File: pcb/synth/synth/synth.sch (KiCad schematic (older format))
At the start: 3 parts, among them J1 Screw_Terminal_01x06, J2 AudioJack2, J3 Conn_02x07_Odd_Even

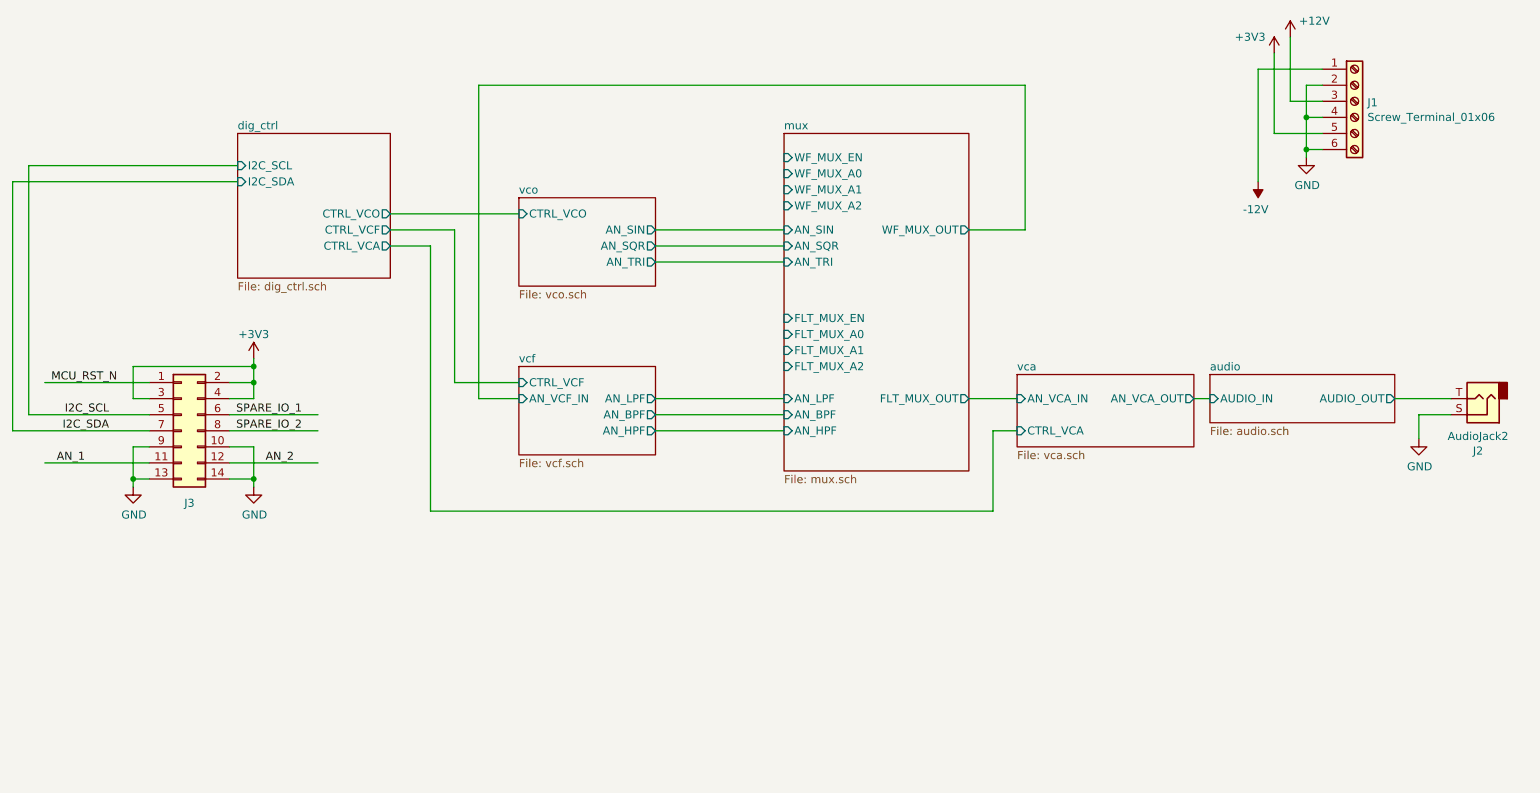
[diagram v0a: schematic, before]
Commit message: inital synth schematic
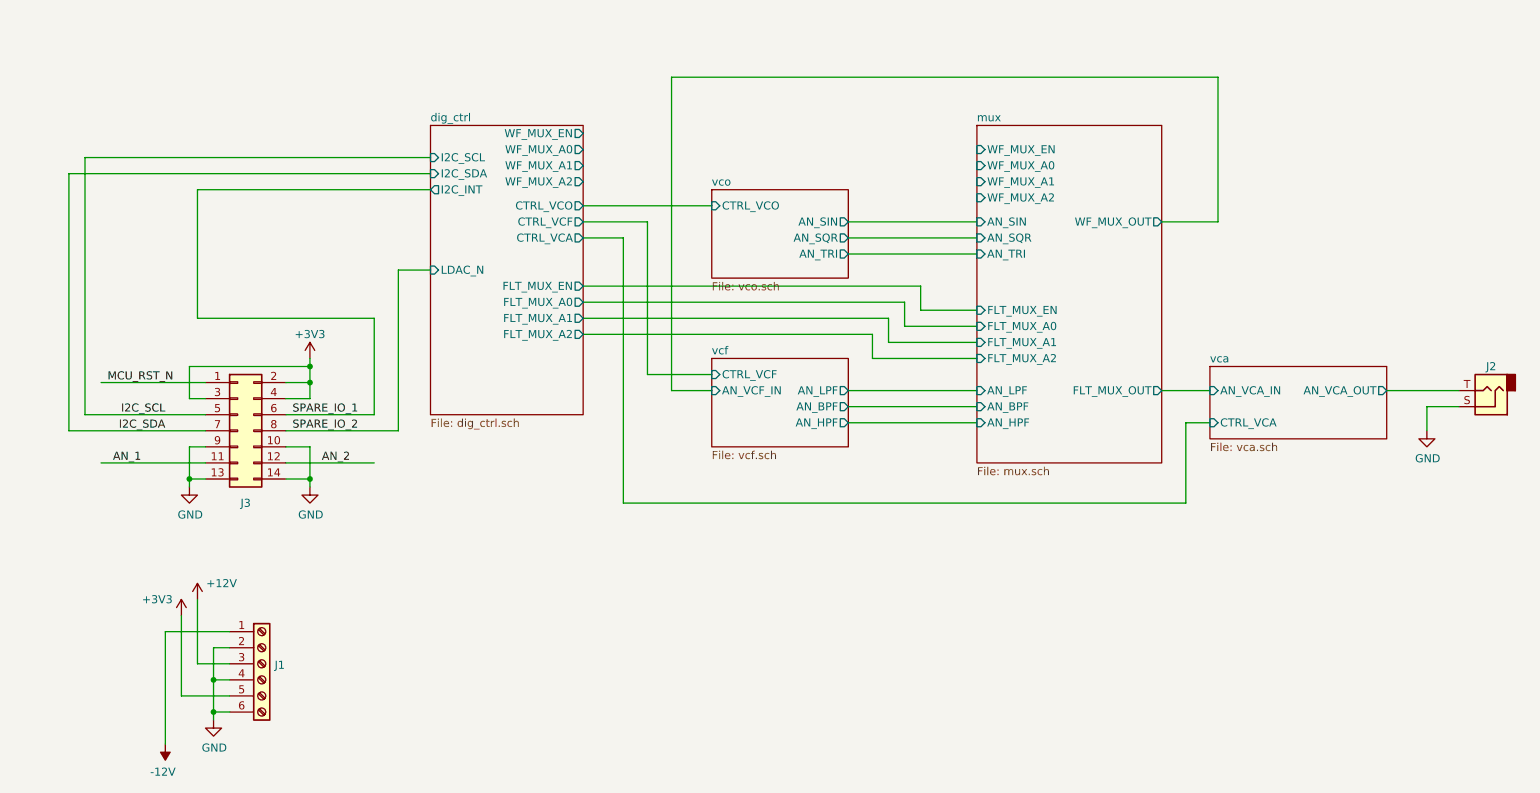
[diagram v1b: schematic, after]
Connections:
- wire segments 64 -> 81
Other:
- moved on the sheet: J1, J2, J3

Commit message: final pcb designs and initial i2c
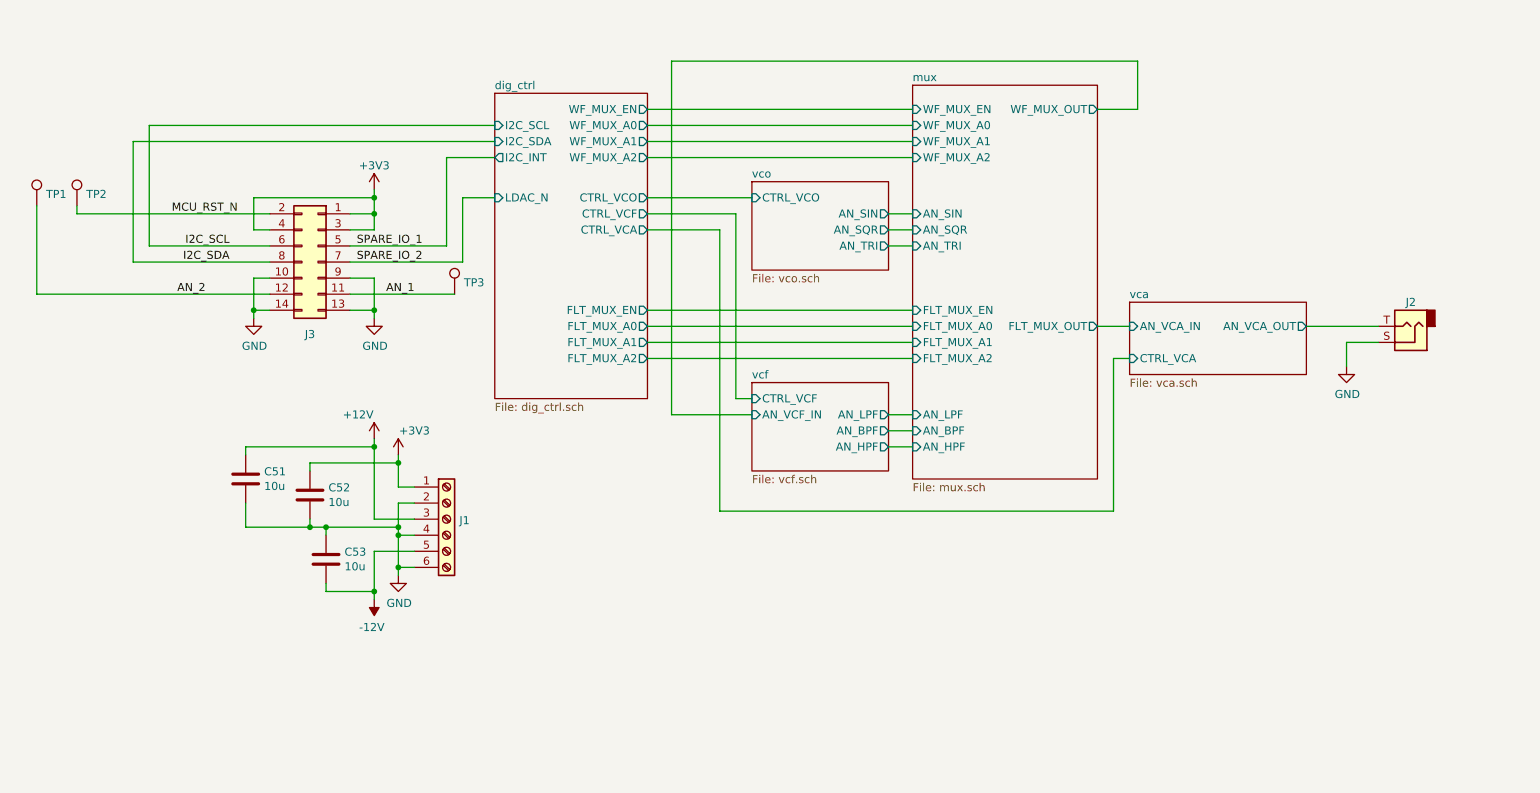
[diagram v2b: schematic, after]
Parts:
- added C51, C52, C53: 10u, Capacitor_SMD:C_0603_1608Metric_Pad1.05x0.95mm_HandSolder, symbol Device:C
- added TP1, TP2, TP3: TestPoint, TestPoint:TestPoint_Pad_1.0x1.0mm, symbol Connector:TestPoint
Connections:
- wire segments 81 -> 93
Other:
- moved on the sheet: J1, J2, J3
